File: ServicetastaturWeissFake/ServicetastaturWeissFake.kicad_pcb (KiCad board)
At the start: 2 copper layers, 153.7 x 57.2 mm, 72 parts, among them J1 Automat, SW1 Gewinn, SW10 Lautspr./, SW11 ↓0,10, SW12 ↑0,10, SW13 ↓Serie, SW14 ↑Serie, SW15 Zeit, SW16 ↑1,-, SW17 ↙0,10, SW18 ↙1,-, SW19 Auszahlquote, SW2 Foul, SW20 ↙5,-, SW21 Münzsp., SW22 Sp.Zähl, SW23 Lampen, SW24 Reset, SW25 Initialisieren, SW26 Münzung, SW27 Ende, SW28 ↑0,10, SW29 ↓Serie, SW3 ↙2,-, SW30 ↑Serie, SW31 ↓1,-, SW32 ↑1,-, SW4 HW-Test, SW5 Münzsp., SW6 Sp.Zähl, SW7 Dauerlauf, SW8 Reset, SW9 Initialisieren, U1 CC56-12CGKWA, U2 CC56-12CGKWA, U3 74LS48, U4 74LS145, U5 74LS48, U6 74LS145

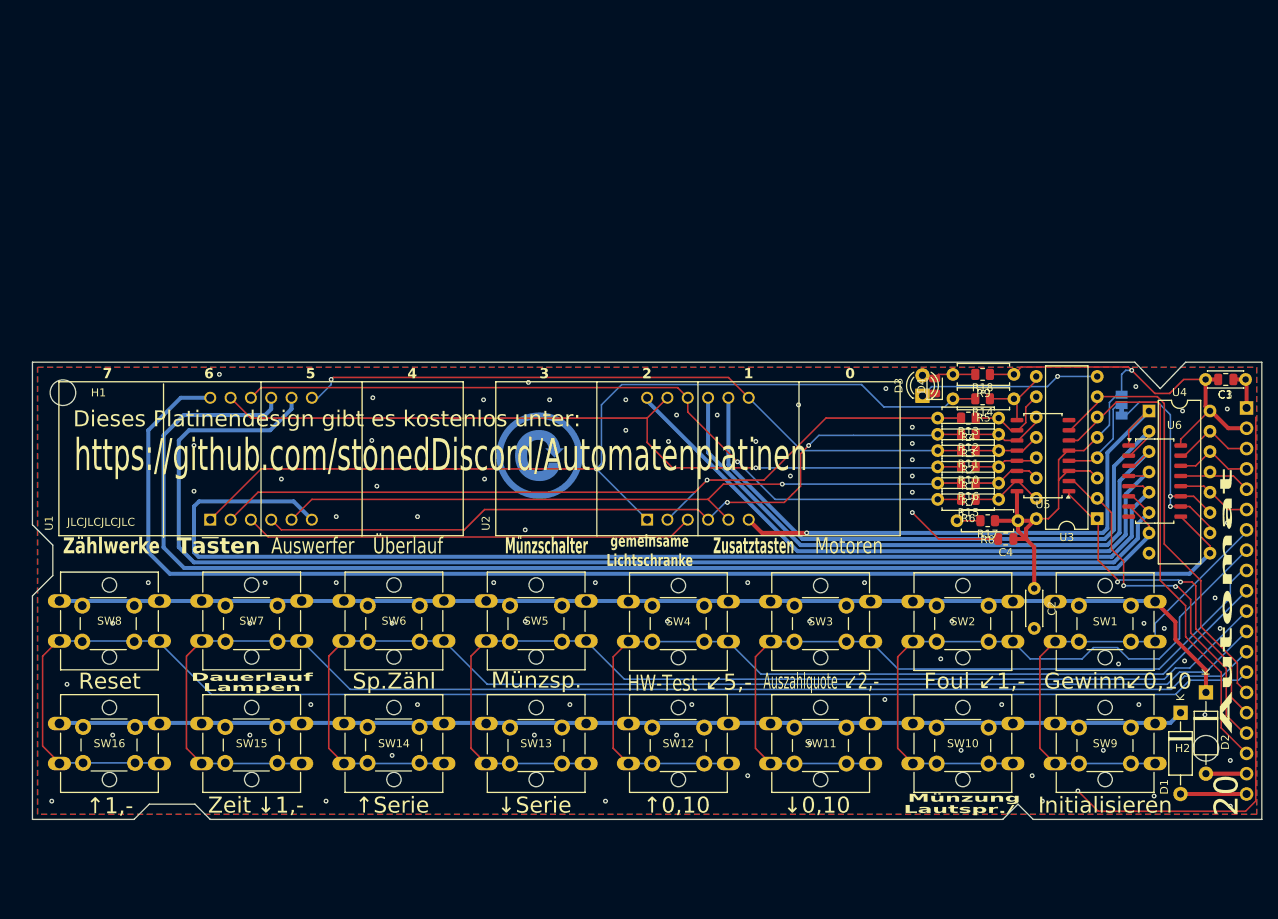
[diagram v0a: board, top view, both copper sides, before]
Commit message: noch eine tastatur
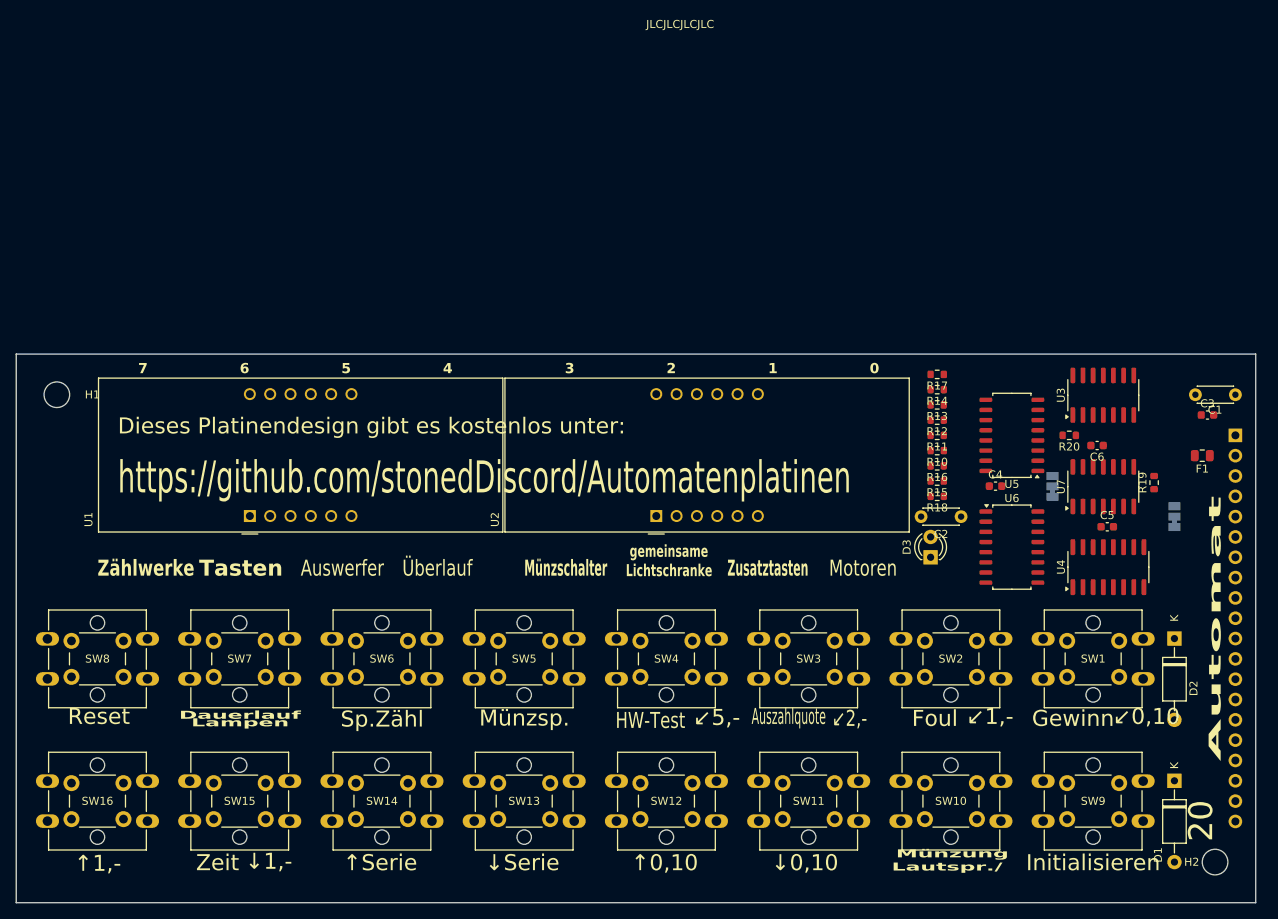
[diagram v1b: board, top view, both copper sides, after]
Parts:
- removed D4: LED, LED_SMD:LED_0805_2012Metric
- removed R1, R2, R3, R4, R5, R6, R7, R8, R9: 470 Ω, Resistor_THT:R_Axial_DIN0207_L6.3mm_D2.5mm_P7.62mm_Horizontal
- removed REF**: KiCad-Logo2_6mm_SilkScreen, Symbol:KiCad-Logo2_6mm_SilkScreen
- removed REF**: OSHW-Logo2_9.8x8mm_SilkScreen, Symbol:OSHW-Logo2_9.8x8mm_SilkScreen
- removed REF**: WEEE-Logo_4.2x6mm_SilkScreen, Symbol:WEEE-Logo_4.2x6mm_SilkScreen
- removed REF**: Symbol_CC-ShareAlike_CopperTop_Big, Symbol:Symbol_CC-ShareAlike_CopperTop_Big
- added C5: 1000pF, Capacitor_SMD:C_0603_1608Metric, F.Cu at (159.2, 47.0)
- added C6: 1000pF, Capacitor_SMD:C_0603_1608Metric, F.Cu at (158.0, 36.8)
- added F1: Fuse, Fuse:Fuse_0805_2012Metric, F.Cu at (171.1, 38.1)
- added JP2: Geschwindigkeit, Jumper:SolderJumper-3_P1.3mm_Bridged12_Pad1.0x1.5mm, B.Cu at (167.6, 45.7)
- added R19: 180 kΩ, Resistor_SMD:R_0603_1608Metric, F.Cu at (165.1, 41.5)
- added R20: 180 kΩ, Resistor_SMD:R_0603_1608Metric, F.Cu at (154.5, 35.6)
- added U7: HEF4093B, Package_SO:SOIC-14_3.9x8.7mm_P1.27mm, F.Cu at (158.8, 42.0)
- C3, C4: footprint Capacitor_SMD:C_0805_2012Metric -> Capacitor_SMD:C_0603_1608Metric
- JP1: value Jumper_3_Bridged12 -> Invers; footprint Jumper:SolderJumper-3_P1.3mm_Bridged12_Pad1.0x1.5mm_NumberLabels -> Jumper:SolderJumper-3_P1.3mm_Bridged12_Pad1.0x1.5mm
- R10, R11, R12, R13, R14, R15, R16, R17, R18: footprint Resistor_SMD:R_0805_2012Metric -> Resistor_SMD:R_0603_1608Metric
- U3: value 74LS48 -> 74LS08; footprint Package_DIP:DIP-16_W7.62mm -> Package_SO:SOIC-14_3.9x8.7mm_P1.27mm
- U4: value 74LS145 -> 4017; footprint Package_DIP:DIP-16_W7.62mm -> Package_SO:SOP-16_3.9x9.9mm_P1.27mm
- moved D3 20.2 mm to (137.2, 50.8)
- moved U4 20.2 mm to (159.4, 52.0), turned to 90 degrees
- moved U6 19.7 mm to (147.3, 49.5)
- moved R17 19.3 mm to (138.0, 27.9)
- moved R18 16.3 mm to (138.0, 43.2)
- moved U3 15.4 mm to (158.8, 30.5), turned to 90 degrees
- moved H2 14.3 mm to (172.7, 88.9)
- moved JP1 13.3 mm to (152.4, 41.9)
- moved C2 12.8 mm to (141.0, 45.7), turned to 180 degrees
- moved D1 8.54 mm to (167.6, 78.7)
- moved D2 7.80 mm to (167.6, 61.0)
- moved SW10 7.35 mm to (133.4, 78.8)
- moved SW9 7.35 mm to (151.2, 78.8)
- moved SW11 7.35 mm to (115.7, 78.8)
- moved SW12 7.35 mm to (97.9, 78.8)
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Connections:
- J1 pad 2: +5V -> Net-(J1-Pin_2)
- JP1 pad 3: +5V -> Net-(JP1-B)
- R10 pad 1: Net-(U3-a) -> Net-(U5-a)
- R11 pad 1: Net-(U3-b) -> Net-(U5-b)
- R12 pad 1: Net-(U3-c) -> Net-(U5-c)
- R13 pad 1: Net-(U3-d) -> Net-(U5-d)
- R14 pad 1: Net-(U3-e) -> Net-(U5-e)
- R15 pad 1: Net-(U3-f) -> Net-(U5-f)
- R16 pad 1: Net-(U3-g) -> Net-(U5-g)
- R17 pad 1: +5V -> Net-(R17-Pad1)
- R17 pad 2: unconnected-(R17-Pad2) -> Net-(U1-DPX)
- U3 pad 10: Net-(U3-d) -> Net-(U3-Pad10)
- U3 pad 11: Net-(U3-c) -> unconnected-(U3-Pad11)
- U3 pad 12: Net-(U3-b) -> unconnected-(U3-Pad12)
- U3 pad 13: Net-(U3-a) -> unconnected-(U3-Pad13)
- U3 pad 14: Net-(U3-g) -> +5V
- U3 pad 2: /A2 -> Net-(U3-Pad2)
- U3 pad 3: +5V -> Net-(U3-Pad10)
- U3 pad 4: Net-(JP1-C) -> /A2
- U3 pad 5: +5V -> /A0
- U3 pad 6: /A3 -> Net-(U3-Pad2)
- U3 pad 7: /A0 -> GND
- U3 pad 8: GND -> Net-(R17-Pad1)
- U3 pad 9: Net-(U3-e) -> /A3
- U4 pad 1: Net-(U2-CC4) -> LED5
- U4 pad 10: Net-(JP1-A) -> LED4
- U4 pad 11: Net-(JP1-A) -> LED9
- U4 pad 12: /S3 -> unconnected-(U4-Cout-Pad12)
- U4 pad 13: /S2 -> GND
- U4 pad 14: /S1 -> Net-(JP2-C)
- U4 pad 15: /S0 -> GND
- U4 pad 2: Net-(U2-CC3) -> LED1
- U4 pad 3: Net-(U2-CC2) -> LED0
- U4 pad 4: Net-(U2-CC1) -> LED2
- U4 pad 5: Net-(U1-CC4) -> LED6
- U4 pad 6: Net-(U1-CC3) -> LED7
- U4 pad 7: Net-(U1-CC2) -> LED3
- U4 pad 9: Net-(U1-CC1) -> LED8
- U5 pad 10: Net-(U3-d) -> Net-(U5-d)
- U5 pad 11: Net-(U3-c) -> Net-(U5-c)
- U5 pad 12: Net-(U3-b) -> Net-(U5-b)
- U5 pad 13: Net-(U3-a) -> Net-(U5-a)
- U5 pad 14: Net-(U3-g) -> Net-(U5-g)
- U5 pad 15: Net-(U3-f) -> Net-(U5-f)
- U5 pad 9: Net-(U3-e) -> Net-(U5-e)
- U6 pad 10: Net-(JP1-A) -> unconnected-(U6-Q8-Pad10)
- U6 pad 11: Net-(JP1-A) -> unconnected-(U6-Q9-Pad11)
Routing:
- net /TS7: track 181.9 -> 0.00 mm
- net Net-(U1-CC1): track 165.7 -> 0.00 mm
- net /TS6: track 164.5 -> 0.00 mm
- net Net-(U1-CC2): track 161.0 -> 0.00 mm
- net Net-(U1-CC3): track 159.6 -> 0.00 mm
- net Net-(D2-K): track 151.4 -> 0.00 mm
- net Net-(U1-CC4): track 149.4 -> 0.00 mm
- net /TS5: track 147.2 -> 0.00 mm
- net Net-(D1-K): track 140.9 -> 0.00 mm
- net /TS4: track 129.9 -> 0.00 mm
- net Net-(U1-e): track 117.5 -> 0.00 mm, vias 1 -> 0
- net /TS3: track 112.6 -> 0.00 mm
- net GND: track 111.9 -> 0.00 mm, vias 84 -> 0
- net Net-(U1-d): track 103.6 -> 0.00 mm, vias 1 -> 0
- net +5V: track 100.8 -> 0.00 mm, vias 1 -> 0
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- removed copper zone on B.Cu, net GND
- removed copper zone on F.Cu, net GND
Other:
- board size 153.7 x 57.2 mm -> 154.9 x 68.6 mm
- board text removed: "Die Produkt ionsdaten gibt es gratis online,"
- board text removed: "Materialwert unter 10€"
